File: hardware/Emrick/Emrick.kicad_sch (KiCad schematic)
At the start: 87 parts, among them J1 LED_STRIP_CONNECTOR, J2 UFL, J3 Conn_02x05_Odd_Even, J4 BATT_CONN, P1 USB_C_Plug_USB2.0, Q1 Q_NPN_DGS, Q2 Q_NPN_DGS, Q3 Q_NPN_DGS, SW1 SW_SPST, SW2 SW_MEC_5E (RESET), U1 74HCT541, U2 CC1310F128RGZR, U3 TPS63020DSJR, U4 CP2102N-A02-GQFN28, U5 MX25R8035FZUIL0, U6 BQ24072RGTR, Y1 24MHz, Y2 32.768kHz

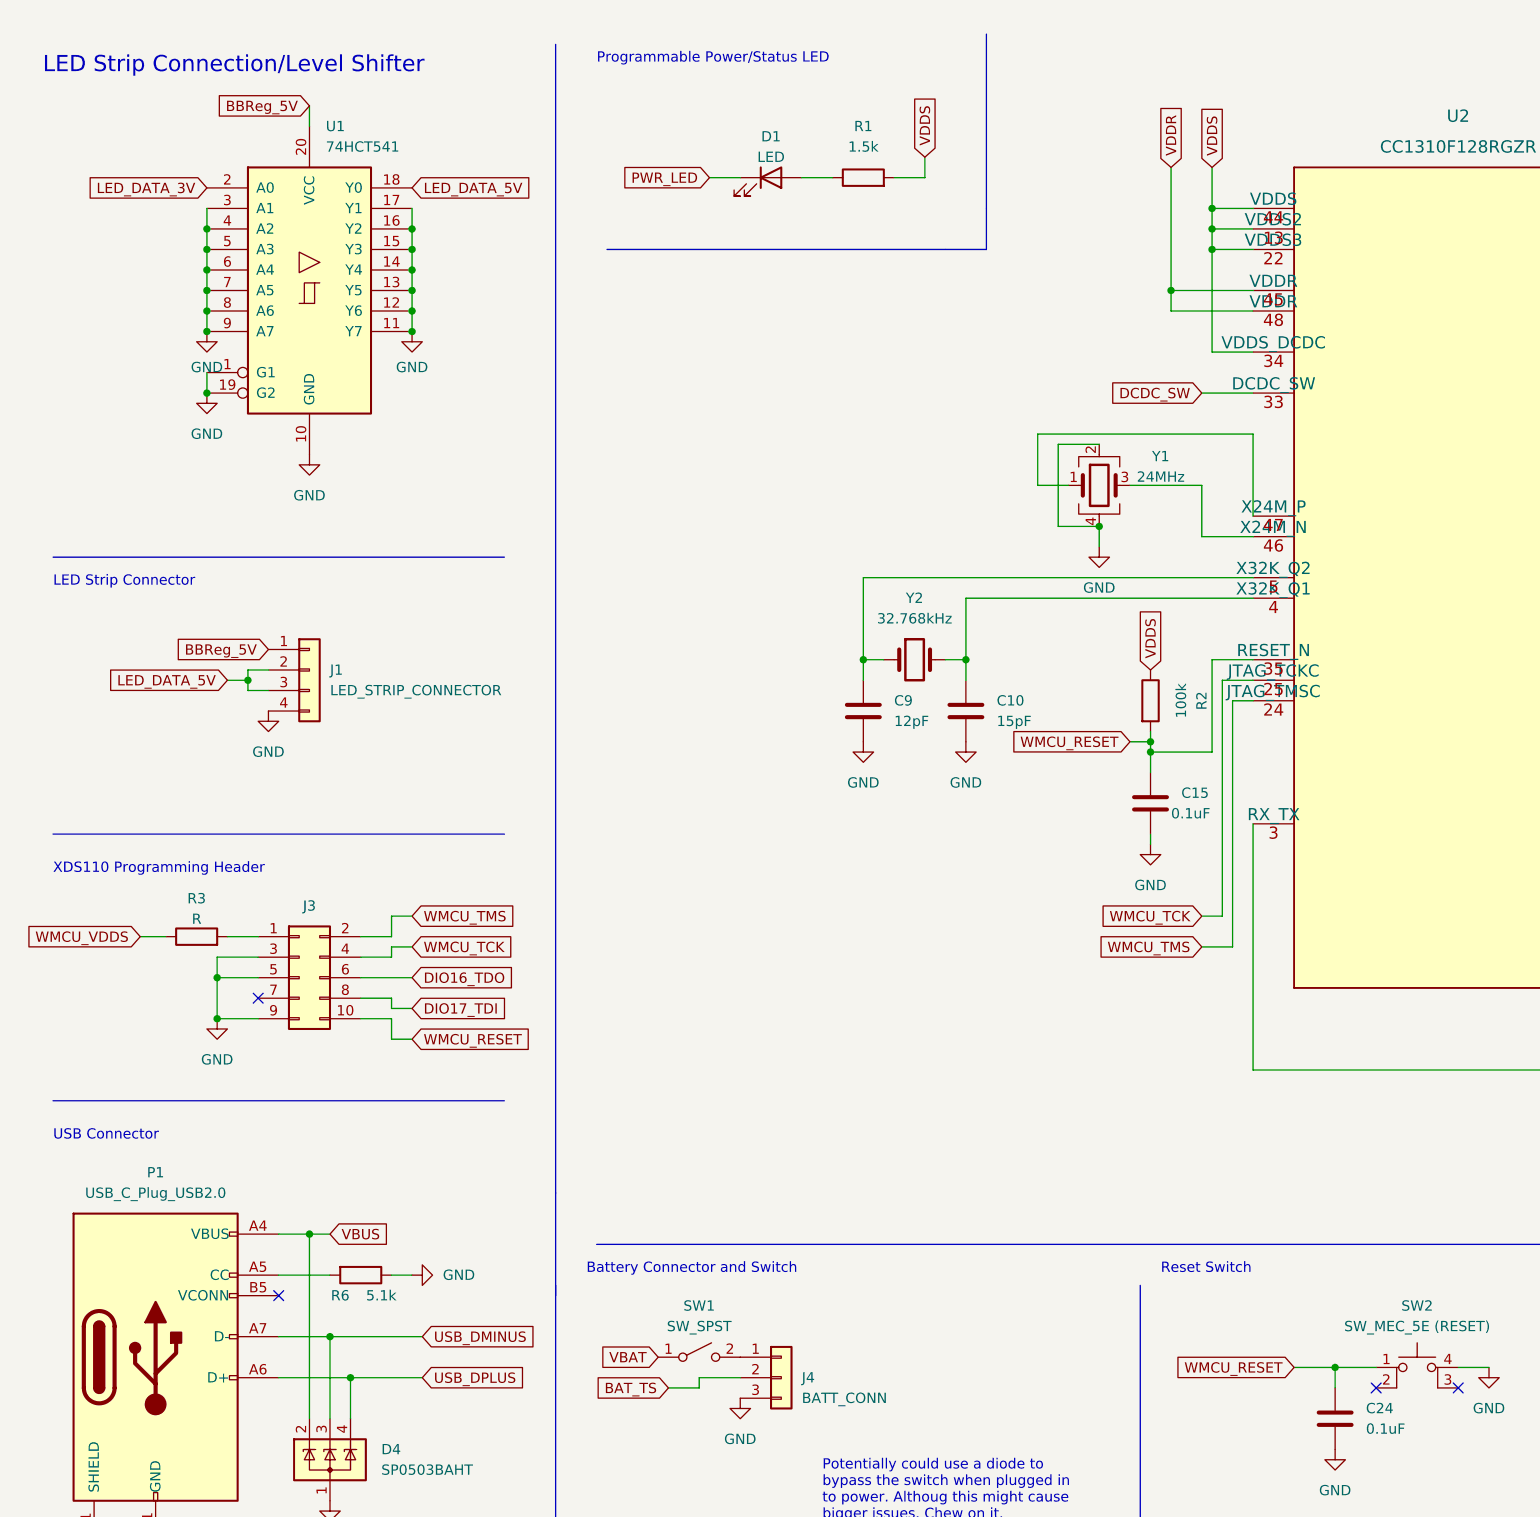
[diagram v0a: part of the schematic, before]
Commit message: added pullup to reset circuitry
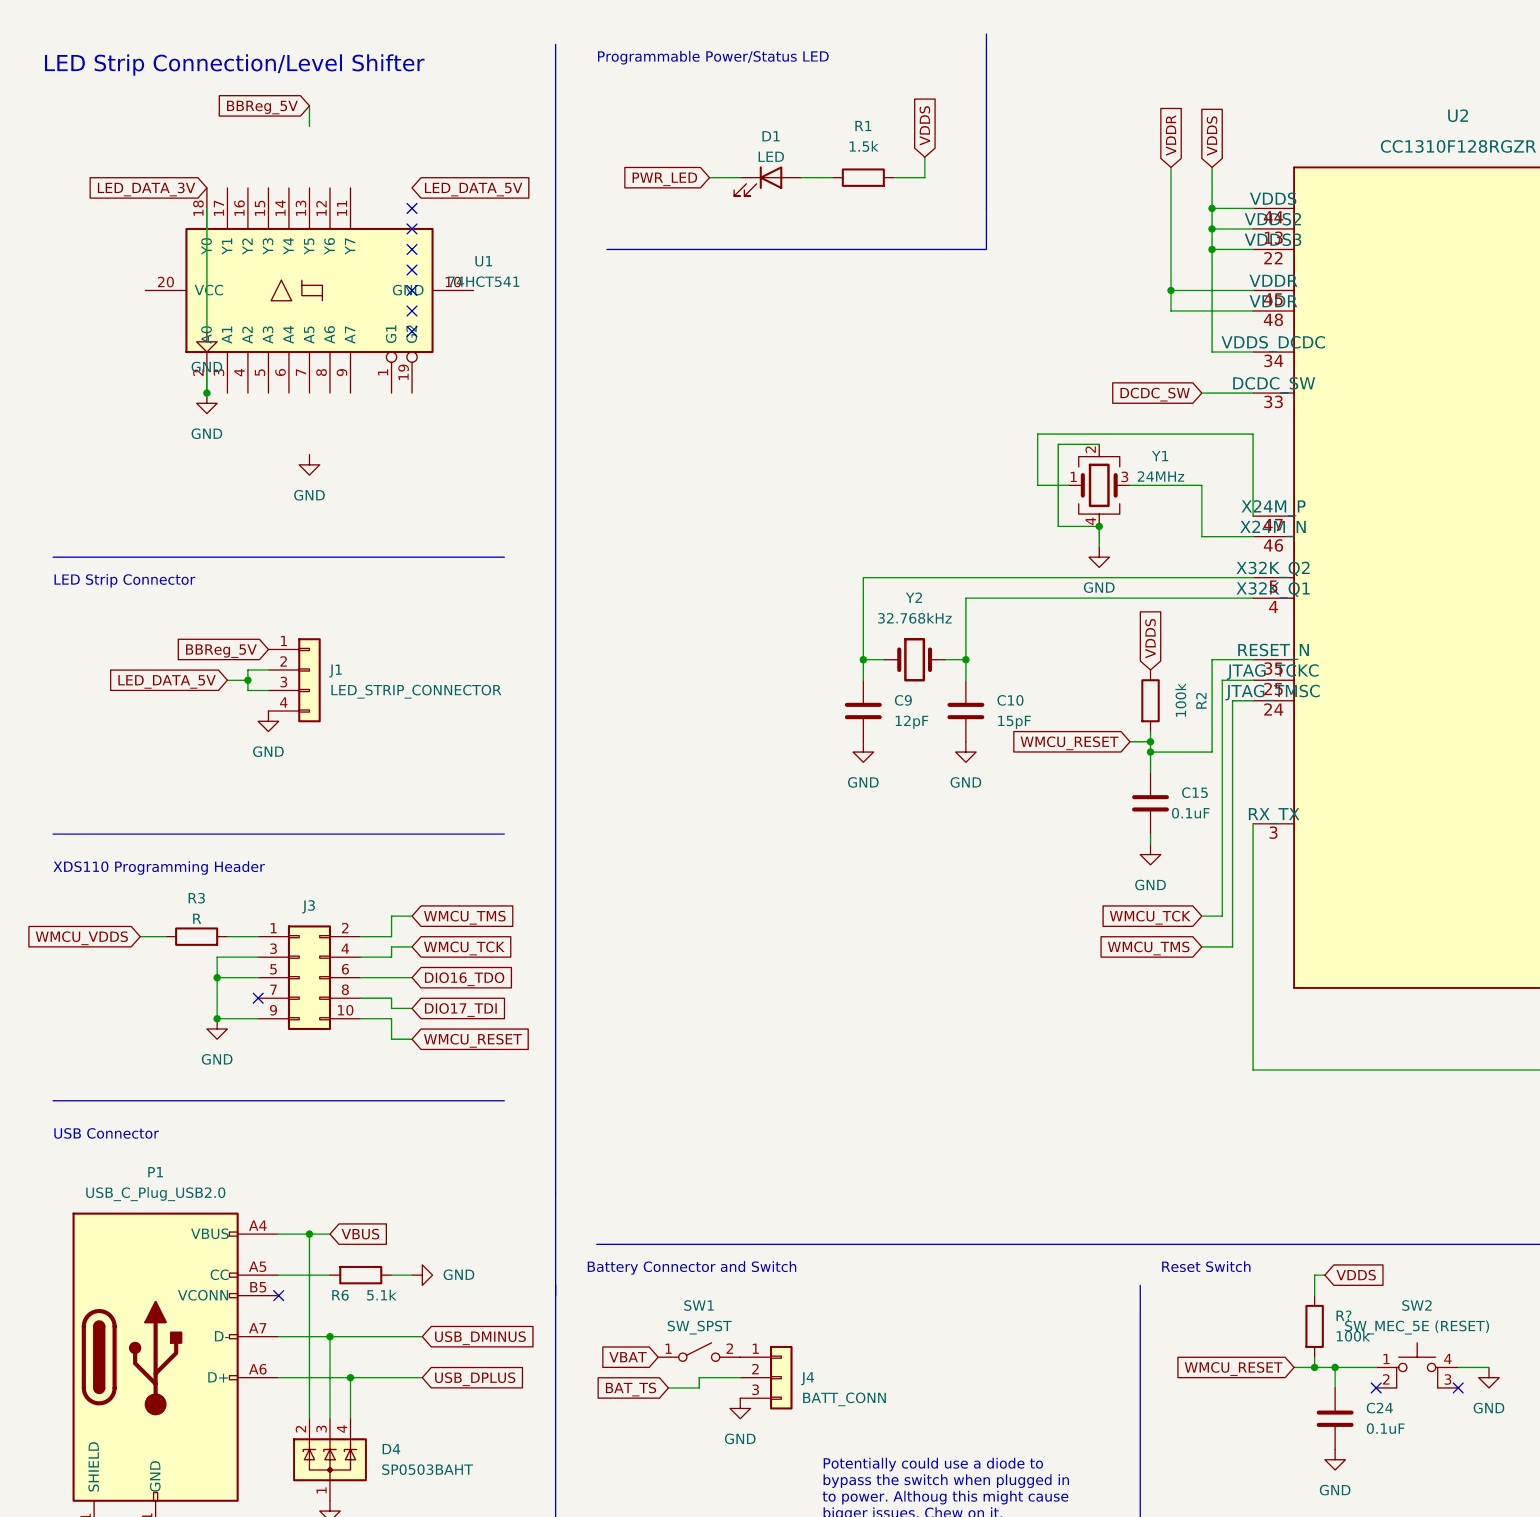
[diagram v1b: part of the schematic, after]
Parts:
- added R?: 100k, symbol Device:R
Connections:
- net BBReg_5V: no longer U1.20 (VCC)
- net GND: now also U1.2 (A0); no longer U1.1 (G1), U1.10 (GND), U1.11 (Y7), U1.12 (Y6), U1.13 (Y5), U1.14 (Y4), U1.15 (Y3), U1.16 (Y2), U1.17 (Y1), U1.19 (G2), U1.3 (A1), U1.4 (A2), U1.5 (A3), U1.6 (A4), U1.7 (A5), U1.8 (A6), U1.9 (A7)
- net LED_DATA_3V: now also U1.18 (Y0); no longer U1.2 (A0)
- net LED_DATA_5V: no longer U1.18 (Y0)
- net VDDS: now also R?.1
- net WMCU_RESET: now also R?.2
- no-connect marks 30 -> 37
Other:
- moved on the sheet: U1

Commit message: Revert "added pullup to reset circuitry"
This reverts commit 352271496a808d8b1eb14a86bebbd64d10ea0814.
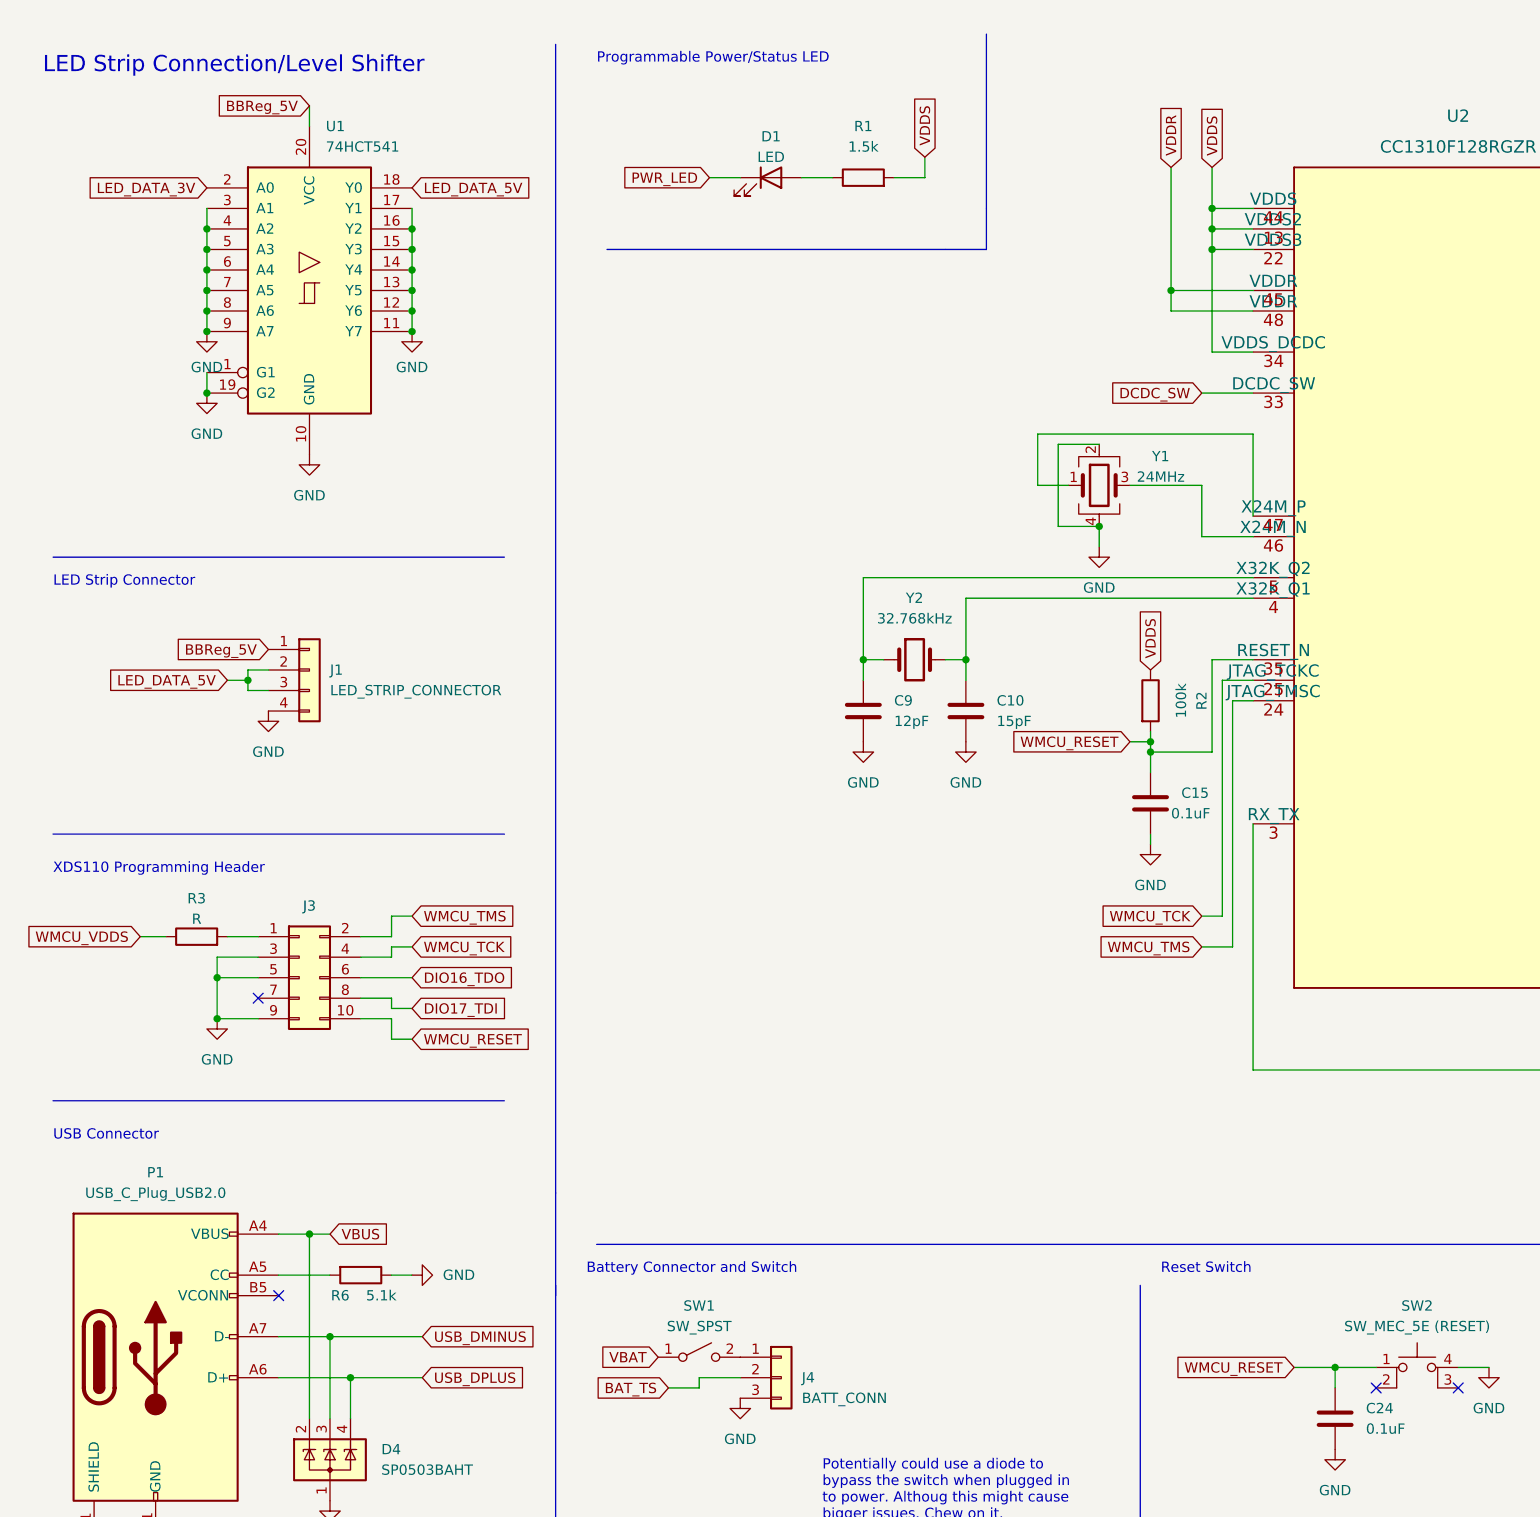
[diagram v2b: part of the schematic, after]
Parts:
- removed R?: 100k, symbol Device:R
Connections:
- net BBReg_5V: now also U1.20 (VCC)
- net GND: now also U1.1 (G1), U1.10 (GND), U1.11 (Y7), U1.12 (Y6), U1.13 (Y5), U1.14 (Y4), U1.15 (Y3), U1.16 (Y2), U1.17 (Y1), U1.19 (G2), U1.3 (A1), U1.4 (A2), U1.5 (A3), U1.6 (A4), U1.7 (A5), U1.8 (A6), U1.9 (A7); no longer U1.2 (A0)
- net LED_DATA_3V: now also U1.2 (A0); no longer U1.18 (Y0)
- net LED_DATA_5V: now also U1.18 (Y0)
- no-connect marks 37 -> 30
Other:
- moved on the sheet: U1
